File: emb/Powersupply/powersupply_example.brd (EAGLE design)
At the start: 84.5 x 76.2 mm, 15 parts, among them IC1 7805TV, IC2 7812TV, IC3 LM2574N-5.0

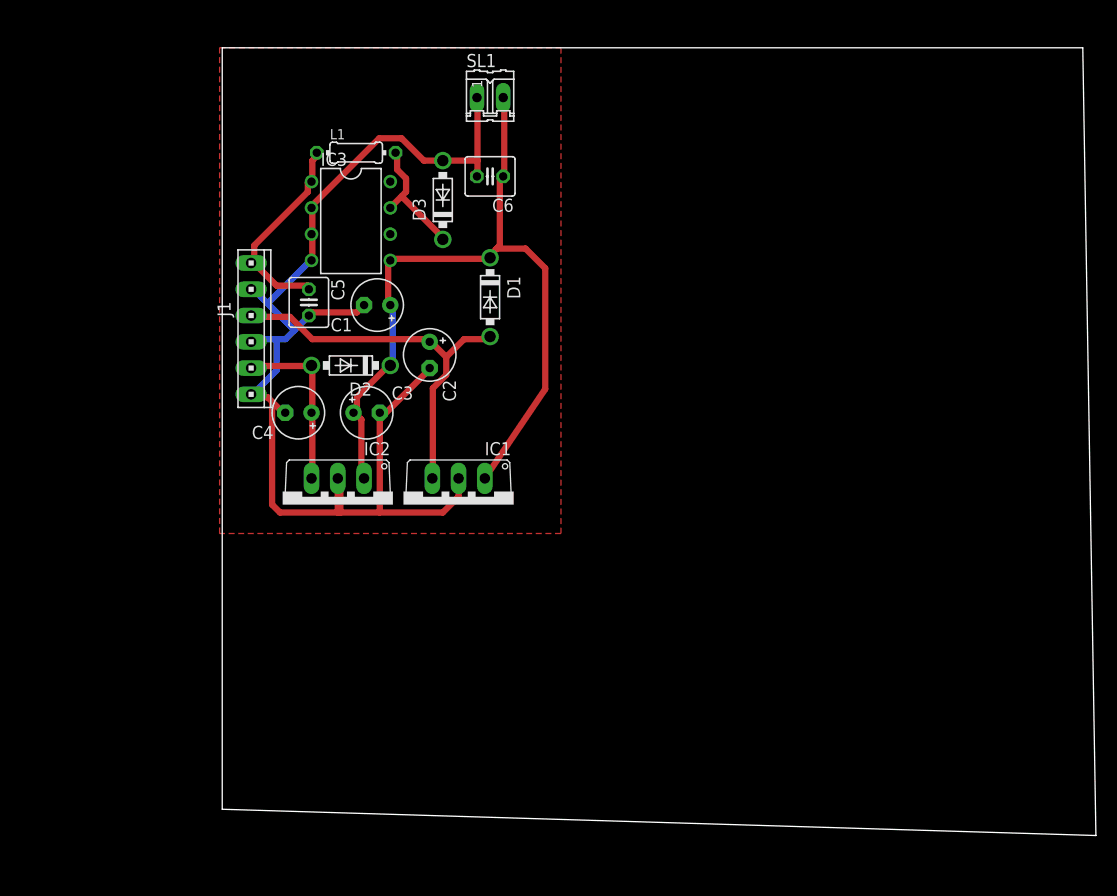
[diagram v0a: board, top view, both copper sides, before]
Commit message: Real powersupply
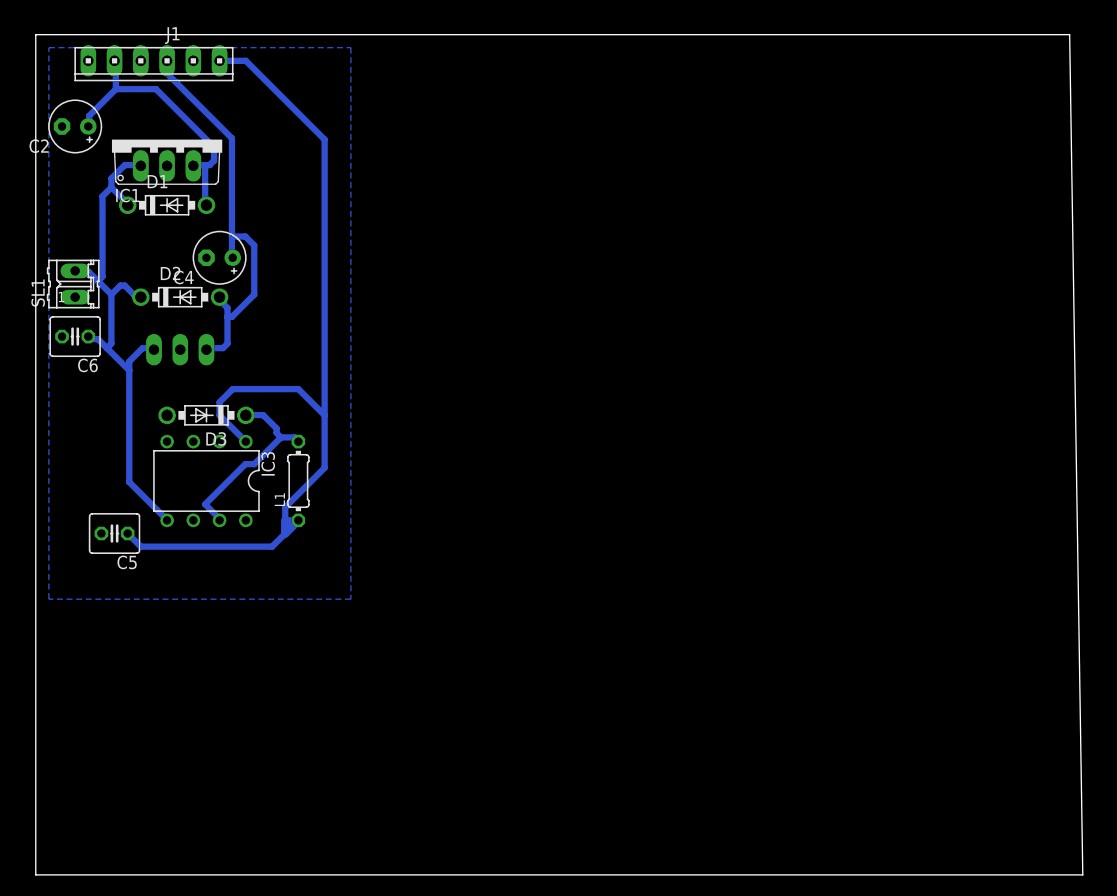
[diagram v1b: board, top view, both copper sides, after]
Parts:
- removed C1, C3: 22µF, rcl:E2,5-5
- moved IC1 45.2 mm to (11.4, 71.1), turned to 0 degrees
- moved SL1 44.0 mm to (2.54, 57.1), turned to 90 degrees
- moved C6 43.0 mm to (2.54, 52.1)
- moved C2 40.8 mm to (2.54, 72.4), turned to 180 degrees
- moved D1 32.5 mm to (11.4, 64.8), turned to 0 degrees
- moved L1 32.2 mm to (24.1, 38.1), turned to 90 degrees
- moved D3 30.9 mm to (15.2, 44.5), turned to 180 degrees
- moved C5 29.2 mm to (6.35, 33.0), turned to 180 degrees
- moved IC3 28.8 mm to (15.2, 38.1), turned to 180 degrees
- moved J1 27.6 mm to (10.2, 78.7), turned to 180 degrees
- moved IC2 19.7 mm to (12.7, 48.3), flipped to the bottom
- moved D2 17.8 mm to (12.7, 55.9), turned to 0 degrees
- moved C4 16.8 mm to (16.5, 59.7)
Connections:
- net 12V: now also J1.4; no longer J1.2
- net 15V: no longer C1.+, C3.+
- net 6V: now also J1.2; no longer J1.4
- net GND: no longer C1.-, C3.-
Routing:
- net GND: track 75.5 -> 0.00 mm
- net 5V: track 20.1 -> 89.0 mm
- net N$1: track 38.4 -> 0.00 mm
- net 12V: track 16.9 -> 39.6 mm
- net 15V: track 77.0 -> 55.2 mm
- net 6V: track 37.9 -> 26.9 mm
- net N$2: track 10.3 -> 0.00 mm
- net N$4: track 12.4 -> 18.5 mm
- added copper zone on layer 16, net GND
- removed copper zone on layer 1, net GND
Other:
- board size 84.5 x 76.2 mm -> 101.3 x 81.3 mm
